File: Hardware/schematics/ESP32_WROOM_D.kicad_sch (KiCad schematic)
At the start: 17 parts, among them J1 Conn_01x02, P1 USB_C_Plug_USB2.0, SW1 BOOT OPTION, U1 exp32wroomd, U2 CH340C, U3 AMS1117-3.3

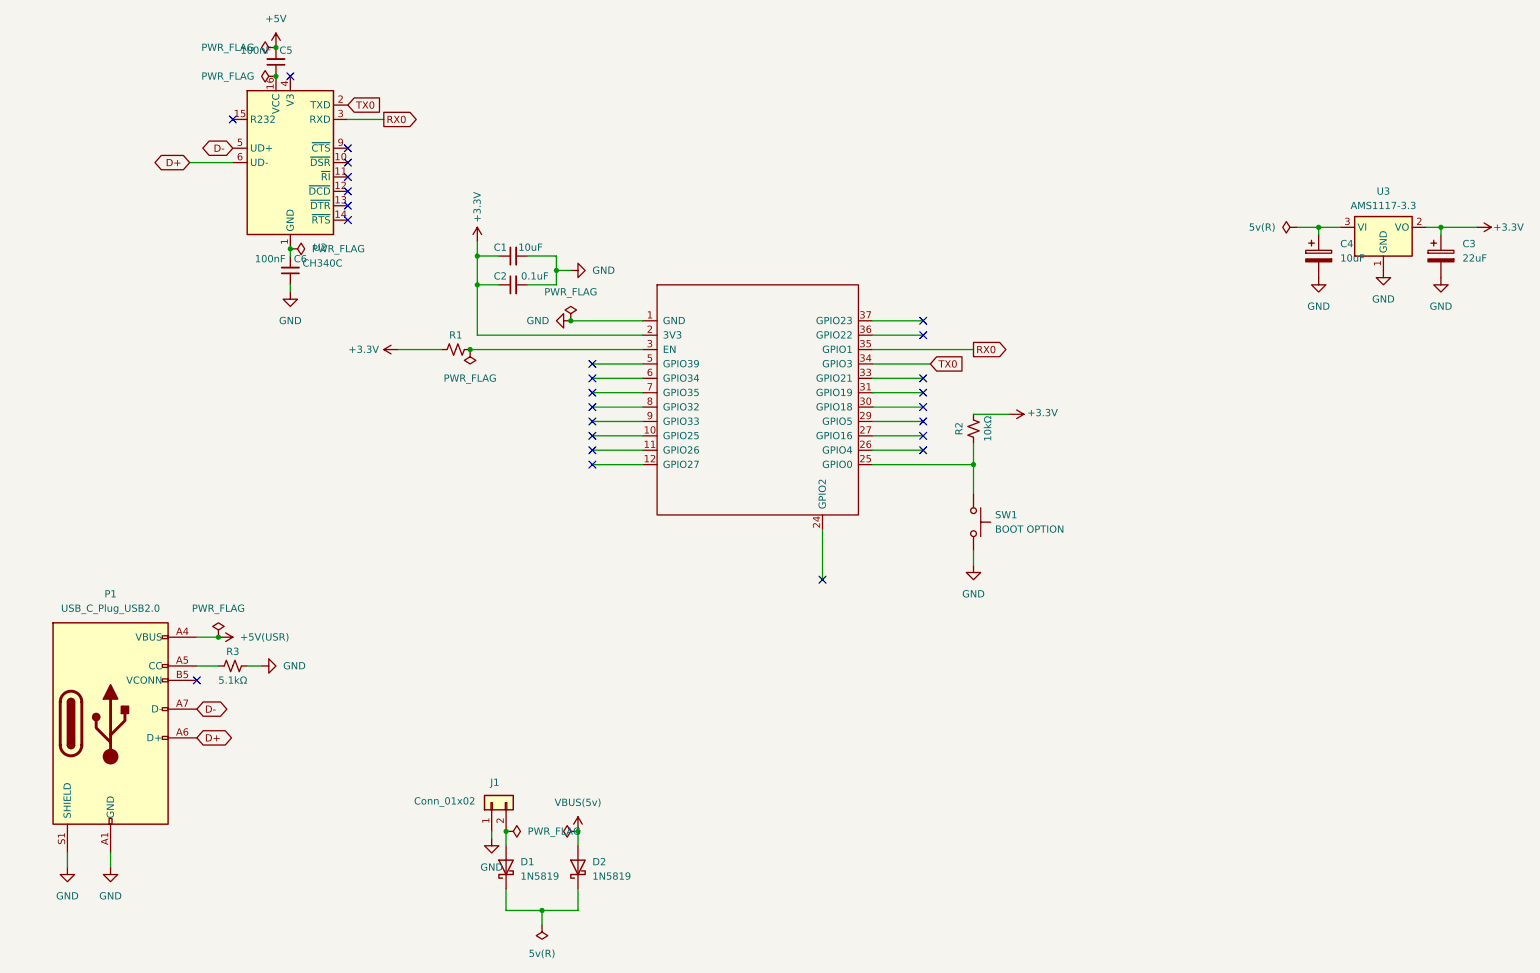
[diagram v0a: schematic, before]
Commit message: Updated schematic
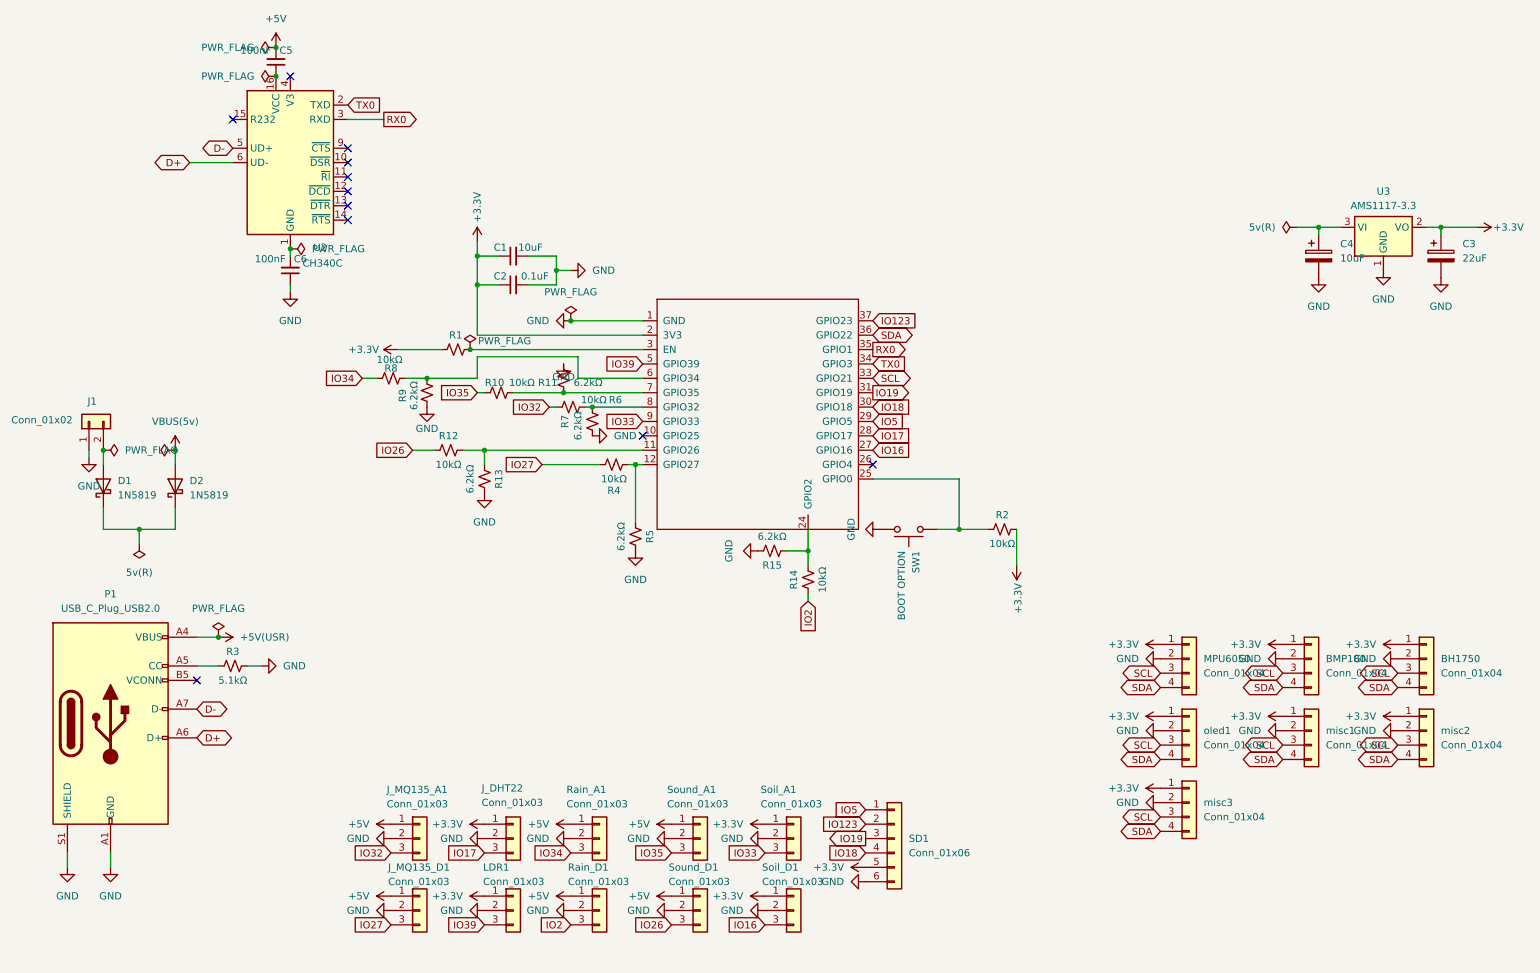
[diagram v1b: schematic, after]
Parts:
- added BH1750, BMP180: Conn_01x04, Connector_PinHeader_2.54mm:PinHeader_1x04_P2.54mm_Vertical, symbol Connector_Generic:Conn_01x04
- added J_DHT22, J_MQ135_A1, J_MQ135_D1, LDR1, Rain_A1, Rain_D1, Soil_A1, Soil_D1, Sound_A1: Conn_01x03, Connector_PinHeader_2.54mm:PinHeader_1x03_P2.54mm_Vertical, symbol Connector_Generic:Conn_01x03
- added MPU6050, misc1, misc2, misc3, oled1: Conn_01x04, Connector_PinHeader_2.54mm:PinHeader_1x03_P2.54mm_Vertical, symbol Connector_Generic:Conn_01x04
- added R10, R12, R14, R4, R6, R8: 10kΩ, Resistor_SMD:R_0603_1608Metric, symbol Device:R_Small_US
- added R11, R13, R15, R5, R7, R9: 6.2kΩ, Resistor_SMD:R_0603_1608Metric, symbol Device:R_Small_US
- added SD1: Conn_01x06, Connector_PinHeader_1.27mm:PinHeader_1x06_P1.27mm_Vertical, symbol Connector_Generic:Conn_01x06
- added Sound_D1: Conn_01x03, Connector_PinHeader_2.54mm:PinHeader_1x04_P2.54mm_Vertical, symbol Connector_Generic:Conn_01x03
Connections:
- net +3.3V: now also BH1750.1 (Pin_1), BMP180.1 (Pin_1), J_DHT22.1 (Pin_1), LDR1.1 (Pin_1), MPU6050.1 (Pin_1), SD1.5 (Pin_5), Soil_A1.1 (Pin_1), Soil_D1.1 (Pin_1), misc1.1 (Pin_1), misc2.1 (Pin_1), misc3.1 (Pin_1), oled1.1 (Pin_1)
- net +5V: now also J_MQ135_A1.1 (Pin_1), J_MQ135_D1.1 (Pin_1), Rain_A1.1 (Pin_1), Rain_D1.1 (Pin_1), Sound_A1.1 (Pin_1), Sound_D1.1 (Pin_1)
- net GND: now also BH1750.2 (Pin_2), BMP180.2 (Pin_2), J_DHT22.2 (Pin_2), J_MQ135_A1.2 (Pin_2), J_MQ135_D1.2 (Pin_2), LDR1.2 (Pin_2), MPU6050.2 (Pin_2), R11.2, R13.2, R15.2, R5.2, R7.2, R9.2, Rain_A1.2 (Pin_2), Rain_D1.2 (Pin_2), SD1.6 (Pin_6), Soil_A1.2 (Pin_2), Soil_D1.2 (Pin_2), Sound_A1.2 (Pin_2), Sound_D1.2 (Pin_2), misc1.2 (Pin_2), misc2.2 (Pin_2), misc3.2 (Pin_2), oled1.2 (Pin_2)
- net at U1.11 (GPIO26): now also R12.2, R13.1
- net at U1.12 (GPIO27): now also R4.2, R5.1
- net at U1.24 (GPIO2): now also R14.2, R15.1
- net IO16: now reaches U1.27 (GPIO16)
- net IO16: now also Soil_D1.3 (Pin_3)
- net IO5: now reaches U1.29 (GPIO5)
- net IO5: now also SD1.1 (Pin_1)
- net IO18: now reaches U1.30 (GPIO18)
- net IO18: now also SD1.4 (Pin_4)
- net IO19: now reaches U1.31 (GPIO19)
- net IO19: now also SD1.3 (Pin_3)
- net SCL: now reaches U1.33 (GPIO21)
- net SCL: now also BH1750.3 (Pin_3), BMP180.3 (Pin_3), MPU6050.3 (Pin_3), misc1.3 (Pin_3), misc2.3 (Pin_3), misc3.3 (Pin_3), oled1.3 (Pin_3)
- net SDA: now reaches U1.36 (GPIO22)
- net SDA: now also BH1750.4 (Pin_4), BMP180.4 (Pin_4), MPU6050.4 (Pin_4), misc1.4 (Pin_4), misc2.4 (Pin_4), misc3.4 (Pin_4), oled1.4 (Pin_4)
- net IO123: now reaches U1.37 (GPIO23)
- net IO123: now also SD1.2 (Pin_2)
- net IO39: now reaches U1.5 (GPIO39)
- net IO39: now also LDR1.3 (Pin_3)
- net at U1.6 (GPIO34): now also R8.2, R9.1
- net at U1.7 (GPIO35): now also R10.2, R11.1
- net at U1.8 (GPIO32): now also R6.2, R7.1
- net IO33: now reaches U1.9 (GPIO33)
- net IO33: now also Soil_A1.3 (Pin_3)
- new net IO17: J_DHT22.3 (Pin_3), U1.28 (GPIO17)
- new net IO2: R14.1, Rain_D1.3 (Pin_3)
- new net IO26: R12.1, Sound_D1.3 (Pin_3)
- new net IO27: J_MQ135_D1.3 (Pin_3), R4.1
- new net IO32: J_MQ135_A1.3 (Pin_3), R6.1
- new net IO34: R8.1, Rain_A1.3 (Pin_3)
- new net IO35: R10.1, Sound_A1.3 (Pin_3)
- no-connect marks 26 -> 11
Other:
- moved on the sheet: D1, D2, J1, R2, SW1
